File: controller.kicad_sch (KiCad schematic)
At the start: 40 parts, among them J10 Conn_01x06_Socket, J5 Conn_01x10_Pin, J6 Conn_01x06_Socket, J7 USB_B, J8 AVR-ISP-6, SW1 SW_SP5T_NR01105, U10 ATmega328PB-A, U11 FT232RL, U12 WE-TVS-82400102, Y1 ECS-2520MV-xxx-xx

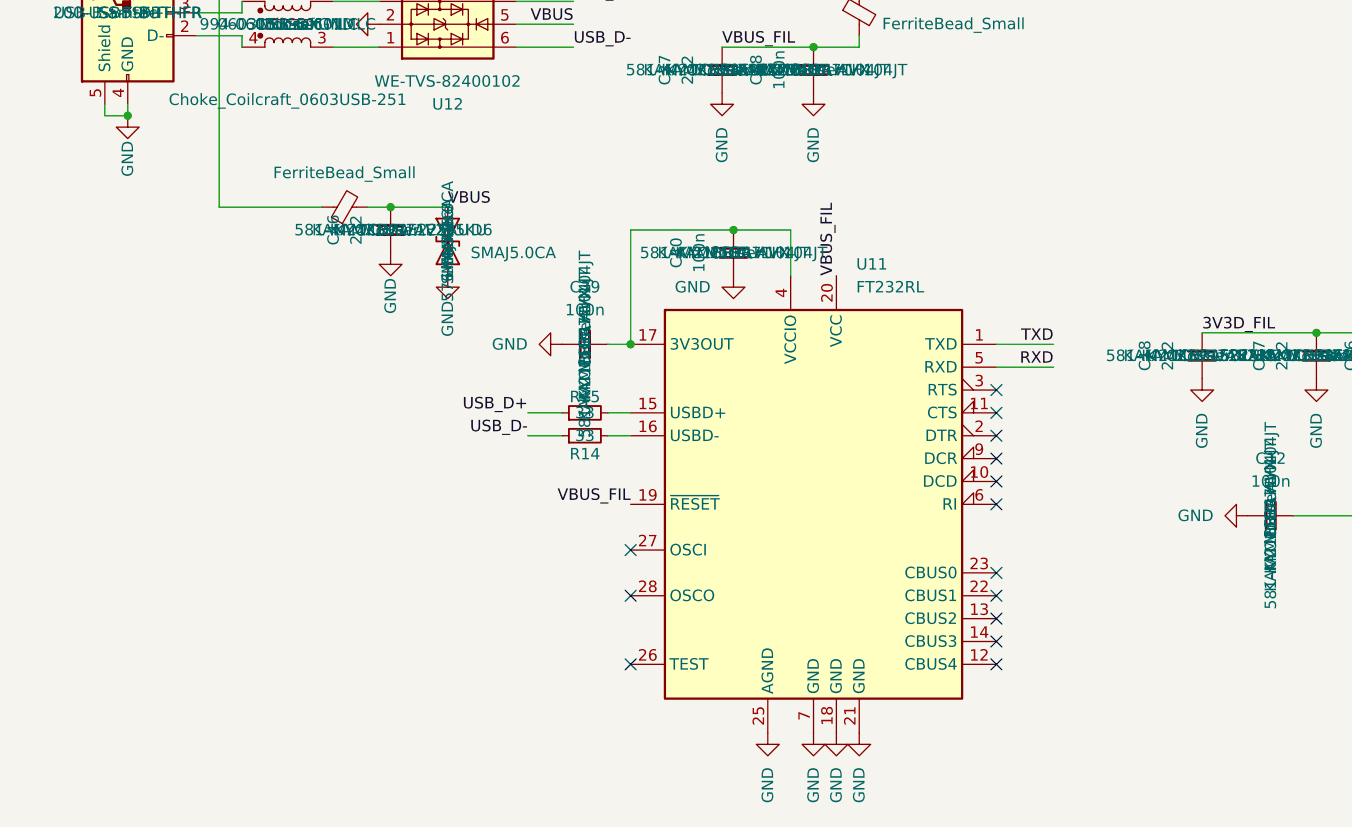
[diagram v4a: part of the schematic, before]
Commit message: es wird nicht besser... Beschriftungen und co. BOM angefangen...
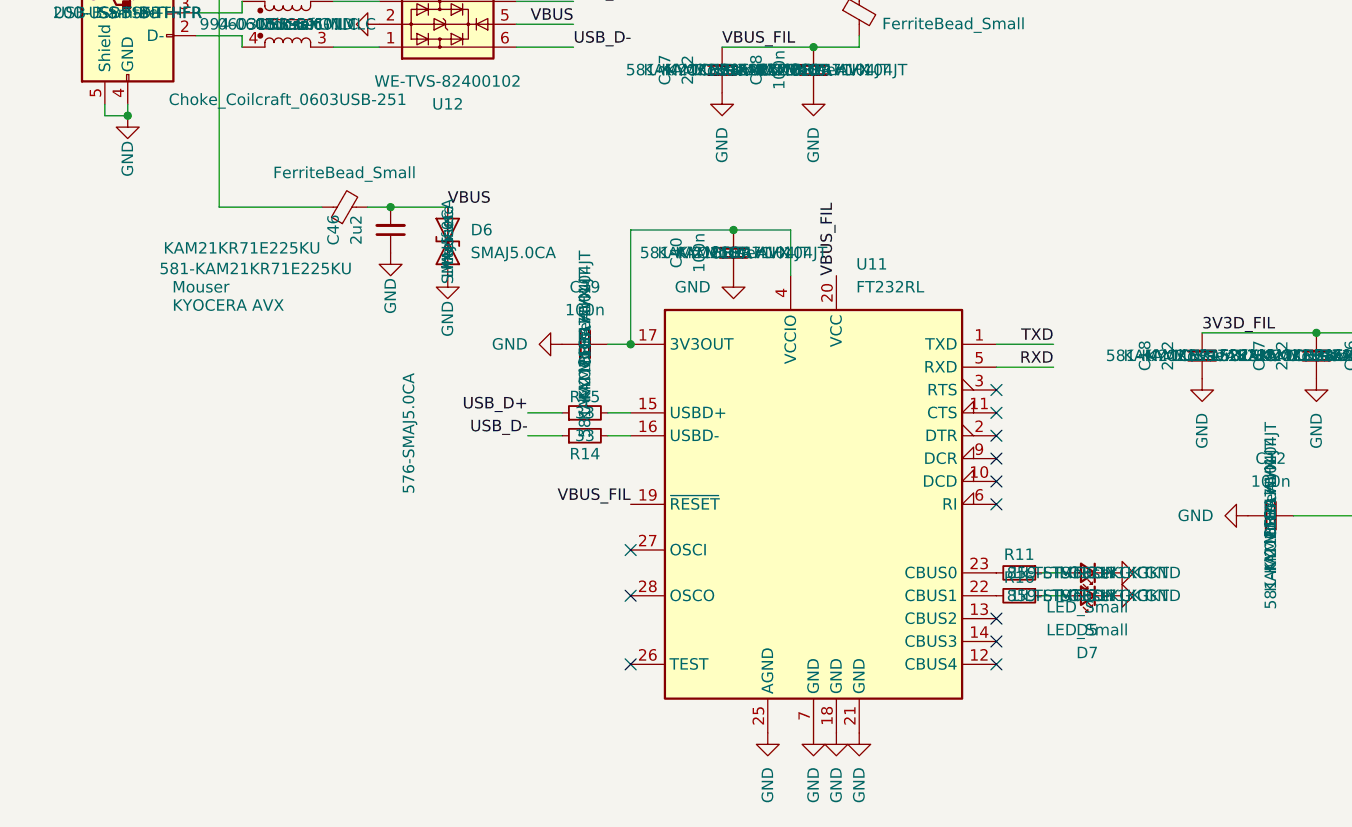
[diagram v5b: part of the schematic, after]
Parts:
- added D5, D7: LED_Small, LED_SMD:LED_0805_2012Metric_Pad1.15x1.40mm_HandSolder, symbol Device:LED_Small
- added R11, R16: 1k, Resistor_SMD:R_0805_2012Metric_Pad1.20x1.40mm_HandSolder, symbol Device:R_Small
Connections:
- net GND: now also D5.1 (K), D7.1 (K)
- net at U11.22 (CBUS1): now also R16.2
- net at U11.23 (CBUS0): now also R11.2
- new net: D7.2 (A), R16.1
- new net: D5.2 (A), R11.1
- no-connect marks 21 -> 19

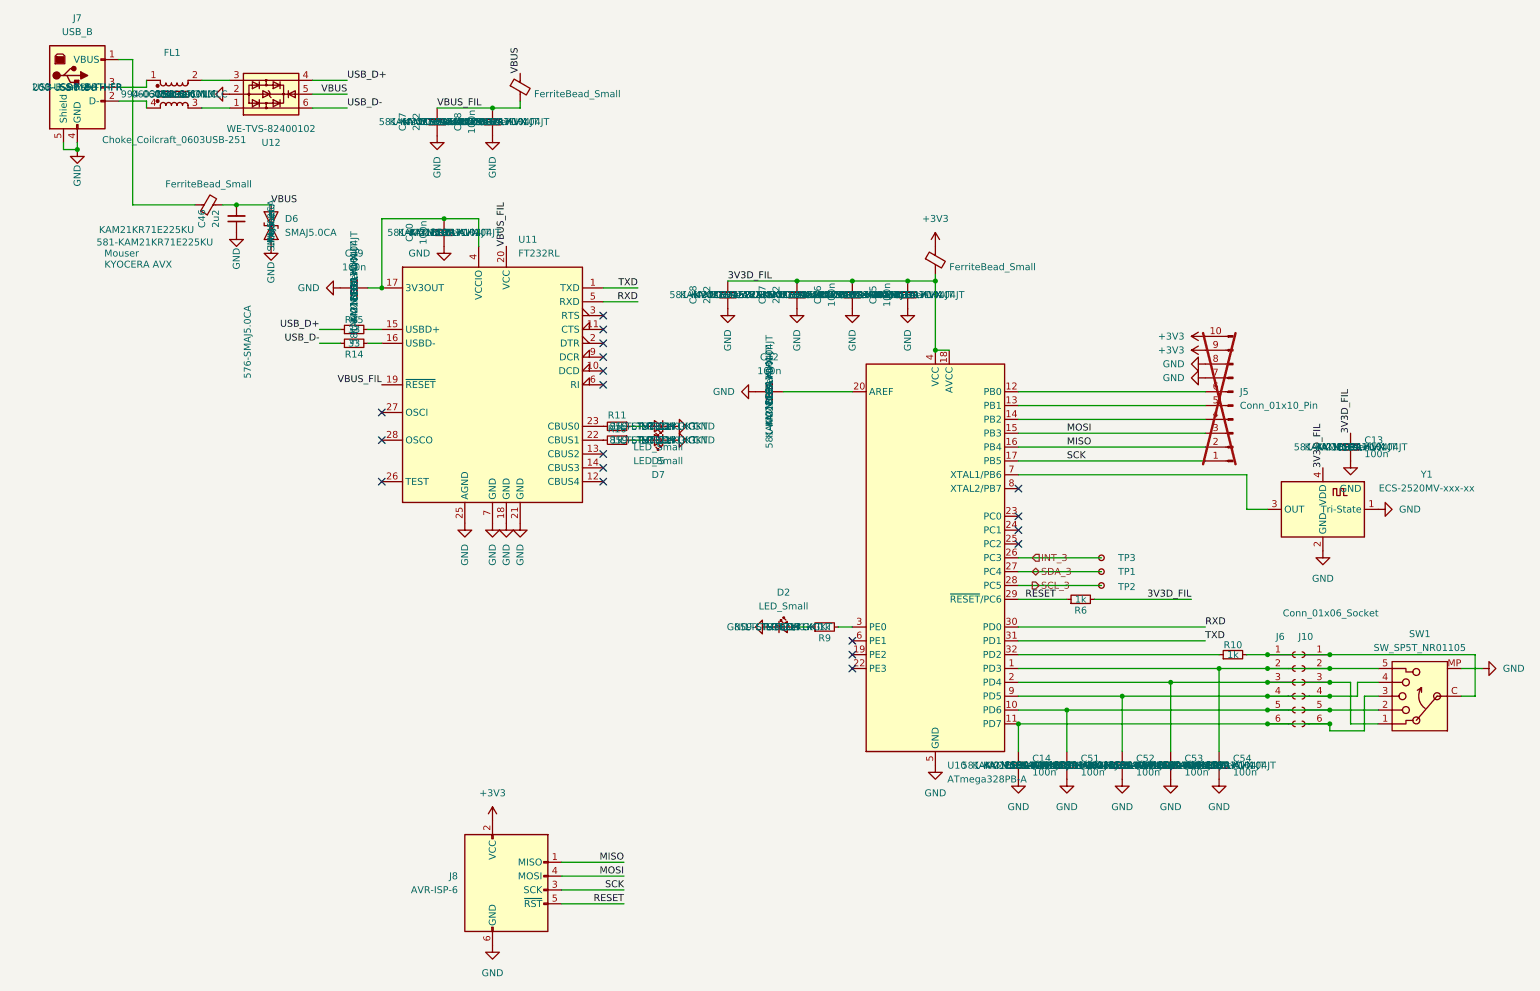
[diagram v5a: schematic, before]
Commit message: BOM...
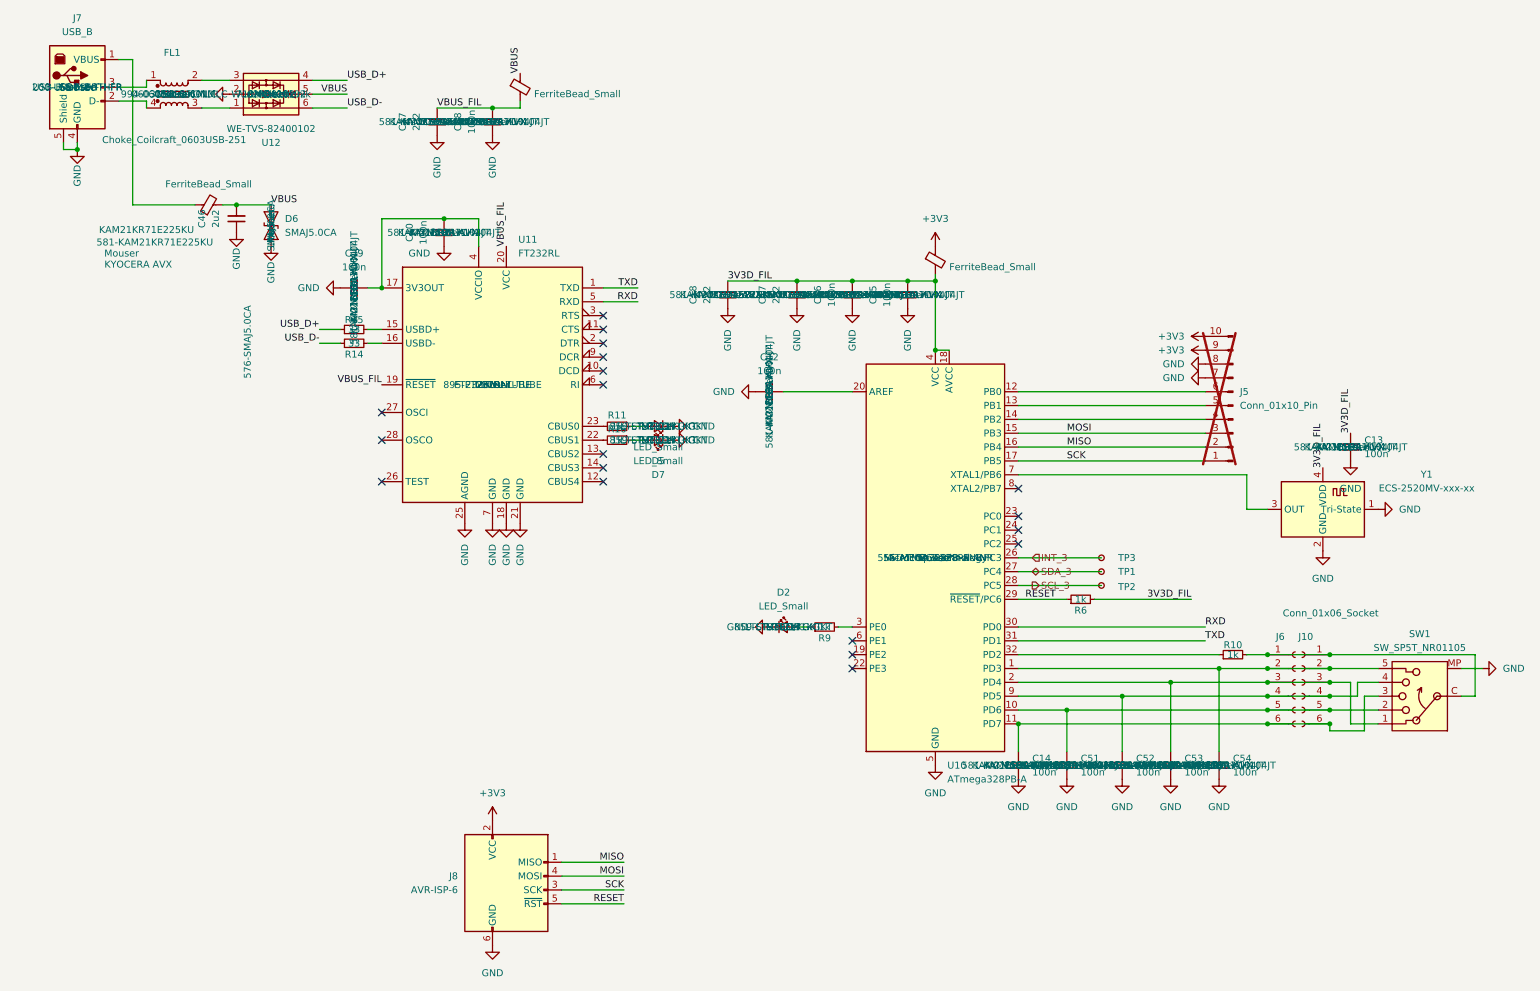
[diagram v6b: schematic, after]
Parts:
- J10: Distributor (none) -> Mouser; Distributor PN (none) -> TC33X-2-103E; Manufacturer (none) -> Adam Tech; Manufacturer PN (none) -> PH1RB-06-UA
- J7: Distributor (none) -> Mouser
- SW1: Distributor (none) -> Mouser; Distributor PN (none) -> 633-NR01105ANG13-2A; Manufacturer (none) -> NKK Switches; Manufacturer PN (none) -> NR01105ANG13-2A
- U10: Distributor (none) -> Mouser; Distributor PN (none) -> 556-ATMEGA328PB-ANR; Manufacturer (none) -> Microchip Technology; Manufacturer PN (none) -> ATMEGA328PB-ANR
- U11: Distributor (none) -> Mouser; Distributor PN (none) -> 895-FT232RNL-TUBE; Manufacturer (none) -> FTDI; Manufacturer PN (none) -> FT232RNL-TUBE
- U12: Distributor (none) -> Mouser; Distributor PN (none) -> 710-82400102; Manufacturer (none) -> Wurth Elektronik; Manufacturer PN (none) -> 82400102
- Y1: Distributor (none) -> Mouser; Distributor PN (none) -> 520-2520MVLC080BNTR3; Manufacturer (none) -> ECS; Manufacturer PN (none) -> ECS-2520MVLC-080-BN-TR3
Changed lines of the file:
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@@
 			)
 		)
+		(property "Distributor" "Mouser"
+			(at 21.59 29.21 0)
+			(effects
+				(font
+					(size 1.27 1.27)
+				)
+			)
+		)
 		(pin "2"
 		)
@@
 			)
 		)
+		(property "Distributor" "Mouser"
+			(at 57.15 30.48 0)
+			(effects
+				(font
+					(size 1.27 1.27)
+				)
+			)
+		)
+		(property "Distributor PN" "710-82400102"
+			(at 57.15 30.48 0)
+			(effects
+				(font
+					(size 1.27 1.27)
+				)
+			)
+		)
+		(property "Manufacturer" "Wurth Elektronik"
+			(at 57.15 30.48 0)
+			(effects
+				(font
+					(size 1.27 1.27)
+				)
+			)
+		)
+		(property "Manufacturer PN" "82400102"
+			(at 57.15 30.48 0)
+			(effects
+				(font
+					(size 1.27 1.27)
+				)
+			)
+		)
 		(pin "5"
 		)
@@
 			)
 		)
-		(property "Manufacturer PN" ""
+		(property "Manufacturer PN" "ECS-2520MVLC-080-BN-TR3 "
 			(at 250.19 106.68 0)
 			(effects
@@
 			)
 		)
-		(property "Manufacturer" ""
+		(property "Manufacturer" "ECS"
 			(at 250.19 106.68 0)
 			(effects
@@
 			)
 		)
-		(property "Distributor" ""
+		(property "Distributor" "Mouser"
 			(at 250.19 106.68 0)
 			(effects
@@
 			)
 		)
-		(property "Distributor PN" ""
+		(property "Distributor PN" " 520-2520MVLC080BNTR3 "
 			(at 250.19 106.68 0)
 			(effects
@@
 			)
 		)
+		(property "Distributor" "Mouser"
+			(at 97.79 83.82 0)
+			(effects
+				(font
+					(size 1.27 1.27)
+				)
+			)
+		)
+		(property "Distributor PN" " 895-FT232RNL-TUBE "
+			(at 97.79 83.82 0)
+			(effects
+				(font
+					(size 1.27 1.27)
+				)
+			)
+		)
+		(property "Manufacturer" "FTDI"
+			(at 97.79 83.82 0)
+			(effects
+				(font
+					(size 1.27 1.27)
+				)
+			)
+		)
+		(property "Manufacturer PN" "FT232RNL-TUBE"
+			(at 97.79 83.82 0)
+			(effects
+				(font
+					(size 1.27 1.27)
+				)
+			)
+		)
 		(pin "21"
 		)
@@
 			)
 		)
+		(property "Distributor" "Mouser"
+			(at 179.07 115.57 0)
+			(effects
+				(font
+					(size 1.27 1.27)
+				)
+			)
+		)
+		(property "Distributor PN" " 556-ATMEGA328PB-ANR"
+			(at 179.07 115.57 0)
+			(effects
+				(font
+					(size 1.27 1.27)
+				)
+			)
+		)
+		(property "Manufacturer" "Microchip Technology "
+			(at 179.07 115.57 0)
+			(effects
+				(font
+					(size 1.27 1.27)
+				)
+			)
+		)
+		(property "Manufacturer PN" "ATMEGA328PB-ANR"
+			(at 179.07 115.57 0)
+			(effects
+				(font
+					(size 1.27 1.27)
+				)
+			)
+		)
 		(pin "5"
 		)
@@
 			)
 		)
-		(property "Manufacturer PN" ""
+		(property "Manufacturer PN" "PH1RB-06-UA"
 			(at 246.38 138.43 0)
 			(effects
@@
 			)
 		)
-		(property "Manufacturer" ""
+		(property "Manufacturer" "Adam Tech "
 			(at 246.38 138.43 0)
 			(effects
@@
 			)
 		)
-		(property "Distributor" ""
+		(property "Distributor" "Mouser"
 			(at 246.38 138.43 0)
 			(effects
@@
 			)
 		)
-		(property "Distributor PN" ""
+		(property "Distributor PN" "TC33X-2-103E"
 			(at 246.38 138.43 0)
 			(effects
@@
 			)
 		)
-		(property "Manufacturer PN" ""
+		(property "Manufacturer PN" "NR01105ANG13-2A"
 			(at 267.97 140.97 0)
 			(effects
@@
 			)
 		)
-		(property "Manufacturer" ""
+		(property "Manufacturer" "NKK Switches"
 			(at 267.97 140.97 0)
 			(effects
@@
 			)
 		)
-		(property "Distributor" ""
+		(property "Distributor" "Mouser"
 			(at 267.97 140.97 0)
 			(effects
@@
 			)
 		)
-		(property "Distributor PN" ""
+		(property "Distributor PN" "633-NR01105ANG13-2A"
 			(at 267.97 140.97 0)
 			(effects
